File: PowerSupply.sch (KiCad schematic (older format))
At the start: 5 parts, among them U401 LM2574N-5.0

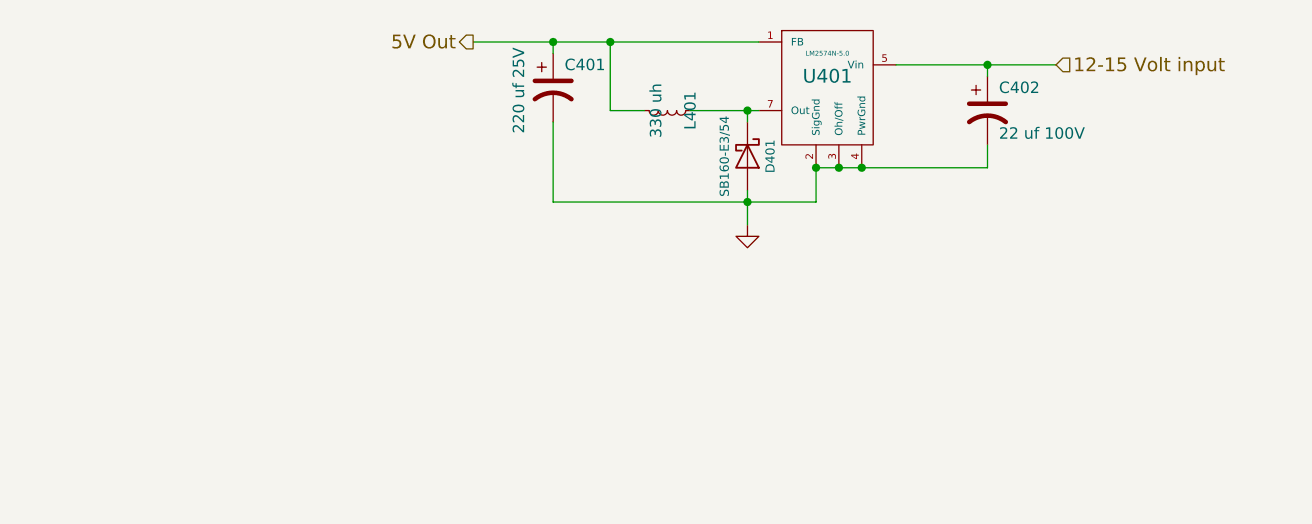
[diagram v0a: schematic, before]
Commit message: Completed initial HW design.
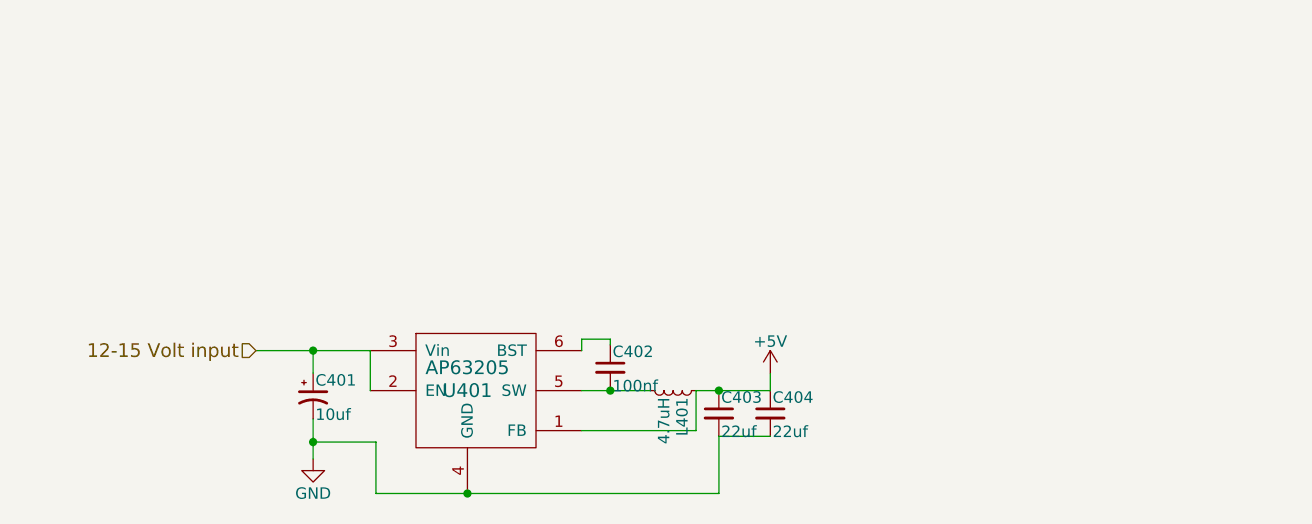
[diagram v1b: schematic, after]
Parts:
- removed C401: 220 uf 25V, Capacitors_THT:CP_Radial_D8.0mm_P3.50mm, symbol CP1
- removed C402: 22 uf 100V, Capacitors_THT:CP_Radial_D8.0mm_P3.50mm, symbol CP1
- removed D401: SB160-E3/54, Diodes_THT:D_DO-41_SOD81_P7.62mm_Horizontal, symbol D_Schottky
- removed U401: LM2574N-5.0, Housings_DIP:DIP-8_W7.62mm, symbol LM2574N-5.0
- added C401: 10uf, Capacitors_SMD:CP_Elec_5x5.3, symbol CP1_Small
- added C402: 100nf, Capacitors_SMD:C_0603, symbol C_Small
- added C403, C404: 22uf, Capacitors_SMD:C_0603, symbol C_Small
- added U401: AP63205, TO_SOT_Packages_SMD:TSOT-23-6_MK06A, symbol AP63205
- L401: value 330 uh -> 4.7uH; footprint PELowProfile:PE-LowProfile -> Inductors_SMD:L_7.3x7.3_H4.5; Mouser Part Number (none) -> 81-B1047AS-4R7NP3; Part Number PE-52627NL -> (none)
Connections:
- net 12-15 Volt input: now also C401.1, U401.2 (EN), U401.3 (Vin)
- net GND: now also C401.2, C403.2, C404.2, U401.4 (GND)
- net +5V: now reaches L401.1
- net +5V: now also C403.1, C404.1, U401.1 (FB)
- net 5V Out: no longer names the net of L401.2
- net 5V Out: now also C402.2, U401.5 (SW)
- new net: C402.1, U401.6 (BST)
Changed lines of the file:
@@
 LIBS:lm2574n-5
 LIBS:sn65hvd233-ht
+LIBS:ap63205
 LIBS:LCC-PNET-Router-cache
 EELAYER 25 0
 EELAYER END
-$Descr A4 11693 8268
+$Descr USLetter 11000 8500
 encoding utf-8
 Sheet 4 4
-Title ""
-Date "4 mar 2019"
-Rev ""
-Comp ""
-Comment1 ""
+Title "ESP32 S3 Multifunction Board Universal Turnout"
+Date ""
+Rev "1.0"
+Comp "Deepwoods Software"
+Comment1 "Power Supply"
 Comment2 ""
 Comment3 ""
@@
 $EndDescr
 $Comp
-L LM2574N-5.0 U401
-U 1 1 63C065F7
-P 5850 3450
-F 0 "U401" H 5850 3500 60  0000 C CNN
-F 1 "LM2574N-5.0" H 5850 3600 21  0000 C CNN
-F 2 "Housings_DIP:DIP-8_W7.62mm" H 5850 3450 60  0001 C CNN
-F 3 "~" H 5850 3450 60  0000 C CNN
-	1    5850 3450
+L +5V #PWR402
+U 1 1 6411E143
+P 5600 4700
+F 0 "#PWR402" H 5600 4550 50  0001 C CNN
+F 1 "+5V" H 5600 4840 50  0000 C CNN
+F 2 "" H 5600 4700 50  0001 C CNN
+F 3 "" H 5600 4700 50  0001 C CNN
+	1    5600 4700
+	1    0    0    -1
+$EndComp
+$Comp
+L AP63205 U401
+U 1 1 6411E144
+P 4275 4775
+F 0 "U401" H 4275 4775 60  0000 C CNN
+F 1 "AP63205" H 4275 4875 60  0000 C CNN
+F 2 "TO_SOT_Packages_SMD:TSOT-23-6_MK06A" H 4275 4775 60  0001 C CNN
+F 3 "" H 4275 4775 60  0001 C CNN
+F 4 "621-AP63205WU-7" H 4275 4775 60  0001 C CNN "Mouser Part Number"
+	1    4275 4775
+	1    0    0    -1
+$EndComp
+$Comp
+L CP1_Small C401
+U 1 1 6411E145
+P 3600 4800
+F 0 "C401" H 3610 4870 50  0000 L CNN
+F 1 "10uf" H 3610 4720 50  0000 L CNN
+F 2 "Capacitors_SMD:CP_Elec_5x5.3" H 3600 4800 50  0001 C CNN
+F 3 "" H 3600 4800 50  0001 C CNN
+F 4 "710-865230542002" H 3600 4800 60  0001 C CNN "Mouser Part Number"
+	1    3600 4800
+	1    0    0    -1
+$EndComp
+$Comp
+L GND #PWR401
+U 1 1 6411E146
+P 3600 5075
+F 0 "#PWR401" H 3600 4825 50  0001 C CNN
+F 1 "GND" H 3600 4925 50  0000 C CNN
+F 2 "" H 3600 5075 50  0001 C CNN
+F 3 "" H 3600 5075 50  0001 C CNN
+	1    3600 5075
+	1    0    0    -1
+$EndComp
+$Comp
+L C_Small C402
+U 1 1 6411E147
+P 4900 4675
+F 0 "C402" H 4910 4745 50  0000 L CNN
+F 1 "100nf" H 4910 4595 50  0000 L CNN
+F 2 "Capacitors_SMD:C_0603" H 4900 4675 50  0001 C CNN
+F 3 "" H 4900 4675 50  0001 C CNN
+F 4 "710-885012206020" H 4900 4675 60  0001 C CNN "Mouser Part Number"
+	1    4900 4675
 	1    0    0    -1
 $EndComp
 $Comp
 L L_Small L401
-U 1 1 63C065F8
-P 5150 3550
-F 0 "L401" H 5150 3650 50  0000 C CNN
-F 1 "330 uh" H 5150 3500 50  0000 C CNN
-F 2 "PELowProfile:PE-LowProfile" H 5150 3550 60  0001 C CNN
-F 3 "~" H 5150 3550 60  0000 C CNN
-F 4 "PE-52627NL" H 5150 3550 60  0001 C CNN "Part Number"
-	1    5150 3550
+U 1 1 6411E148
+P 5175 4775
+F 0 "L401" H 5205 4815 50  0000 L CNN
+F 1 "4.7uH" H 5205 4735 50  0000 L CNN
+F 2 "Inductors_SMD:L_7.3x7.3_H4.5" H 5175 4775 50  0001 C CNN
+F 3 "" H 5175 4775 50  0001 C CNN
+F 4 "81-B1047AS-4R7NP3" H 5175 4775 60  0001 C CNN "Mouser Part Number"
+	1    5175 4775
 	0    1    1    0
 $EndComp
-Wire Wire Line
-	4900 3550 4900 3250
-Wire Wire Line
-	4300 3250 5550 3250
 $Comp
-L CP1 C401
-U 1 1 63C065F9
-P 4650 3450
-F 0 "C401" H 4700 3550 50  0000 L CNN
-F 1 "220 uf 25V" V 4500 3250 50  0000 L CNN
-F 2 "Capacitors_THT:CP_Radial_D8.0mm_P3.50mm" H 4650 3450 60  0001 C CNN
-F 3 "~" H 4650 3450 60  0000 C CNN
-F 4 "710-860080474010" H 4650 3450 60  0001 C CNN "Part Number"
-	1    4650 3450
-	1    0    0    -1
-$EndComp
-Connection ~ 4900 3250
-$Comp
-L GND #PWR028
-U 1 1 63C065FA
-P 5500 4050
-F 0 "#PWR028" H 5500 4050 30  0001 C CNN
-F 1 "GND" H 5500 3980 30  0001 C CNN
-F 2 "" H 5500 4050 60  0000 C CNN
-F 3 "" H 5500 4050 60  0000 C CNN
-	1    5500 4050
+L C_Small C403
+U 1 1 6411E149
+P 5375 4875
+F 0 "C403" H 5385 4945 50  0000 L CNN
+F 1 "22uf" H 5385 4795 50  0000 L CNN
+F 2 "Capacitors_SMD:C_0603" H 5375 4875 50  0001 C CNN
+F 3 "" H 5375 4875 50  0001 C CNN
+F 4 "603-CC0603MRX6S5B226" H 5375 4875 60  0001 C CNN "Mouser Part Number"
+	1    5375 4875
 	1    0    0    -1
 $EndComp
 Wire Wire Line
-	6550 3800 5800 3800
-Connection ~ 5900 3800
-Connection ~ 5800 3800
+	3350 4600 3850 4600
+Wire Wire Line
+	3850 4600 3850 4775
+Wire Wire Line
+	3600 4700 3600 4600
+Connection ~ 3600 4600
+Wire Wire Line
+	3600 4900 3600 5075
+Wire Wire Line
+	4775 4550 4775 4600
+Wire Wire Line
+	4775 4550 4900 4550
+Wire Wire Line
+	4900 4550 4900 4575
+Wire Wire Line
+	4775 4775 5075 4775
+Connection ~ 4900 4775
+Wire Wire Line
+	5275 4775 5600 4775
 $Comp
-L CP1 C402
-U 1 1 63C065FB
-P 6550 3550
-F 0 "C402" H 6600 3650 50  0000 L CNN
-F 1 "22 uf 100V" H 6600 3450 50  0000 L CNN
-F 2 "Capacitors_THT:CP_Radial_D8.0mm_P3.50mm" H 6550 3550 60  0001 C CNN
-F 3 "~" H 6550 3550 60  0000 C CNN
-F 4 "667-ECA-1VM220I" H 6550 3550 60  0001 C CNN "Part Number"
-	1    6550 3550
+L C_Small C404
+U 1 1 6411E14A
+P 5600 4875
+F 0 "C404" H 5610 4945 50  0000 L CNN
+F 1 "22uf" H 5610 4795 50  0000 L CNN
+F 2 "Capacitors_SMD:C_0603" H 5600 4875 50  0001 C CNN
+F 3 "" H 5600 4875 50  0001 C CNN
+F 4 "603-CC0603MRX6S5B226" H 5600 4875 60  0001 C CNN "Mouser Part Number"
+	1    5600 4875
 	1    0    0    -1
 $EndComp
+Connection ~ 5375 4775
 Wire Wire Line
-	6150 3350 6850 3350
+	5600 4775 5600 4700
 Wire Wire Line
-	6550 3700 6550 3800
-Connection ~ 6000 3800
-$Comp
-L D_Schottky D401
-U 1 1 63C065FC
-P 5500 3750
-F 0 "D401" H 5500 3850 40  0000 C CNN
-F 1 "SB160-E3/54" H 5500 3650 40  0000 C CNN
-F 2 "Diodes_THT:D_DO-41_SOD81_P7.62mm_Horizontal" H 5500 3750 60  0001 C CNN
-F 3 "~" H 5500 3750 60  0000 C CNN
-F 4 "750-SB160E-G" H 5500 3750 60  0001 C CNN "Mouser Part Number"
-	1    5500 3750
-	0    1    1    0
-$EndComp
+	3875 5225 5375 5225
 Wire Wire Line
-	5250 3550 5550 3550
-Connection ~ 5500 3550
+	3875 5225 3875 5000
 Wire Wire Line
-	5800 3800 5800 3950
+	3875 5000 3600 5000
+Connection ~ 3600 5000
 Wire Wire Line
-	5800 3950 4650 3950
+	5275 4950 4775 4950
 Wire Wire Line
-	5500 3900 5500 4050
+	5275 4950 5275 4775
 Wire Wire Line
-	4650 3950 4650 3600
-Connection ~ 5500 3950
-Text HLabel 4300 3250 0    60   Output ~ 0
-5V Out
-Connection ~ 4650 3250
-Text HLabel 6850 3350 2    60   Input ~ 0
+	5600 4975 5375 4975
+Wire Wire Line
+	5375 4975 5375 5225
+Connection ~ 4275 5225
+Text HLabel 3350 4600 0    60   Input ~ 0
 12-15 Volt input
-Connection ~ 6550 3350
-Wire Wire Line
-	4650 3300 4650 3250
-Wire Wire Line
-	4900 3550 5050 3550
-Wire Wire Line
-	5500 3600 5500 3550
-Wire Wire Line
-	6550 3400 6550 3350
 $EndSCHEMATC
